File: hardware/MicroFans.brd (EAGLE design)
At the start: 100 x 80 mm, 29 parts, among them IC4 ATMEGA328P, IC7 OPA4251UA, J1 COMPUTER-PERIPHERAL-POWERVERT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, Y1 20Mhz

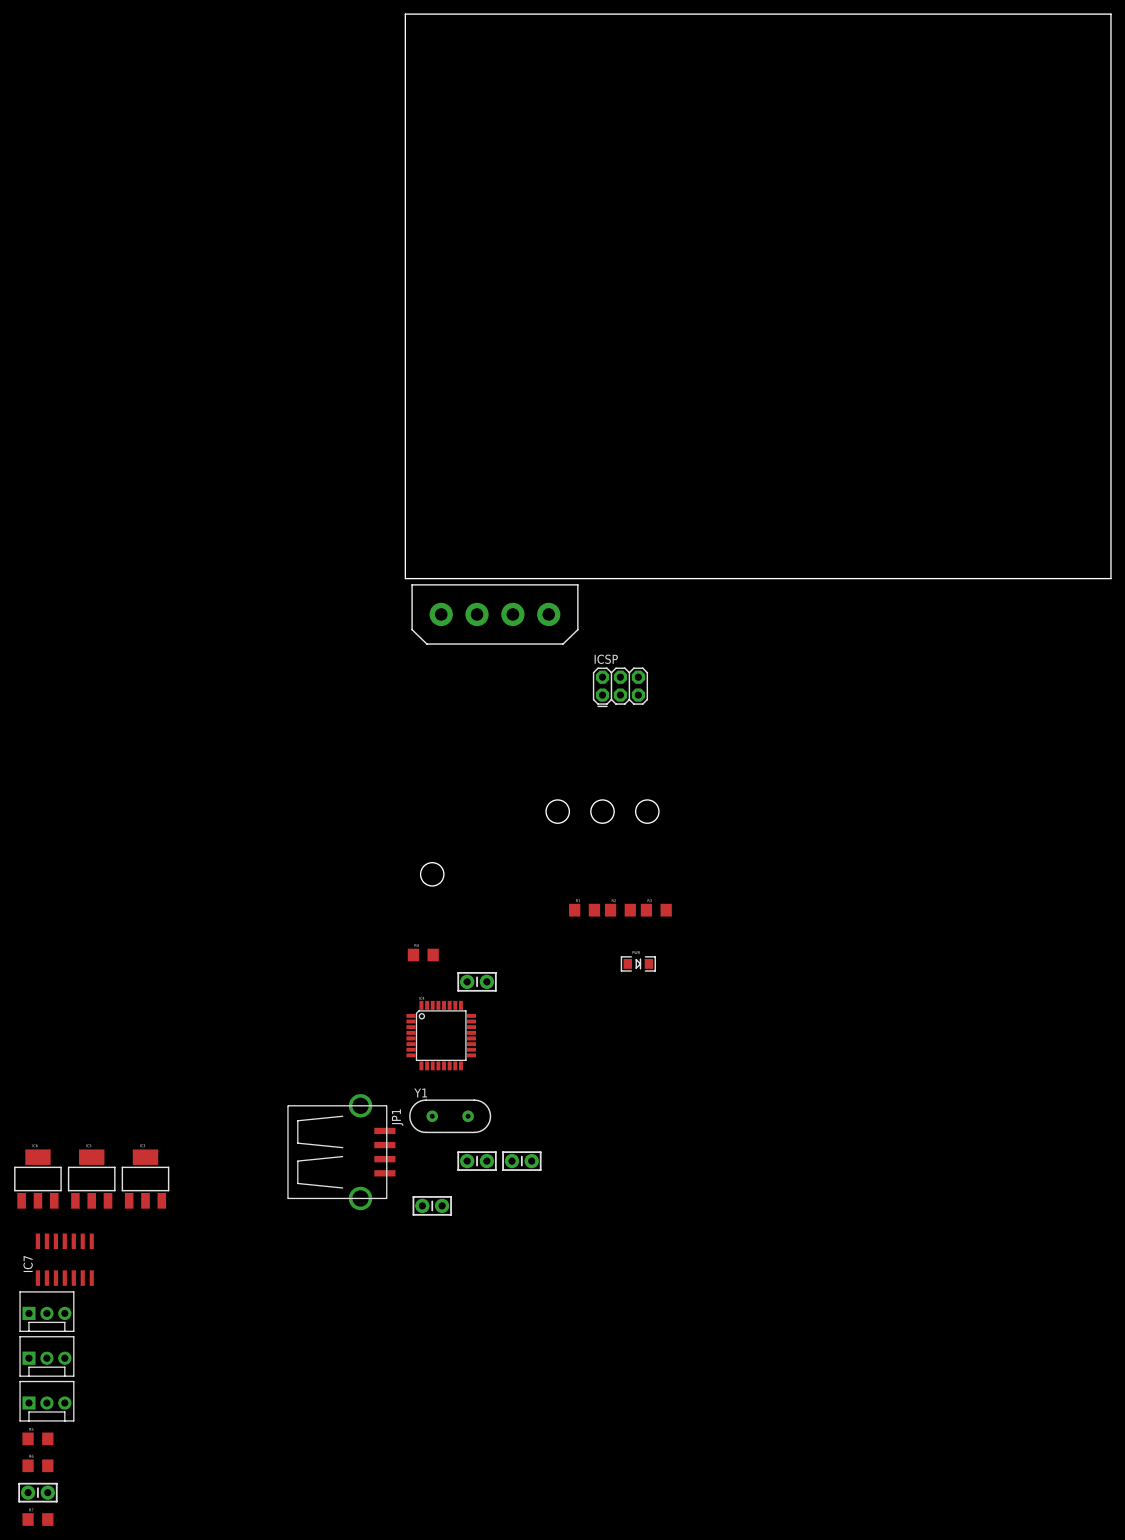
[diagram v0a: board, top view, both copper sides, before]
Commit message: Update board
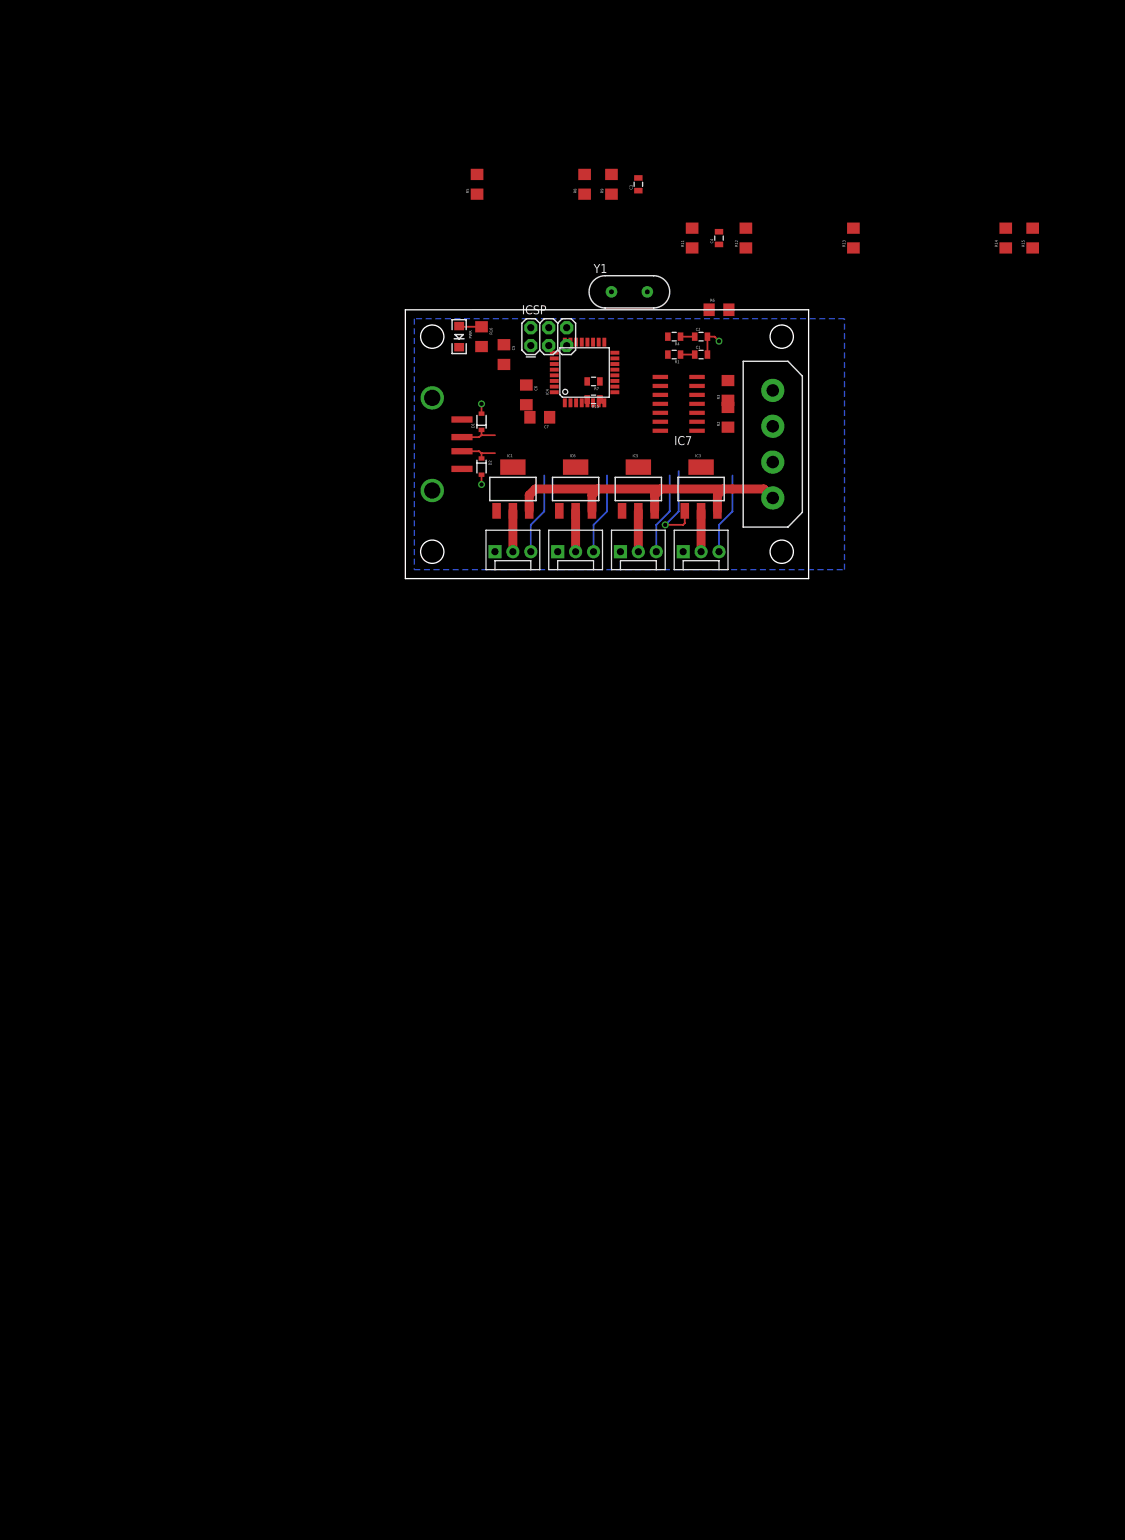
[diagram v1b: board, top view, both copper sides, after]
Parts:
- added C3: 1uF, SparkFun-Capacitors:0805
- added C7: 0.1uF, SparkFun-Passives:1206
- added D1, D2: 3V6, SparkFun-DiscreteSemi:SOD-323
- added IC1: (no value), SparkFun-PowerIC:SOT223
- added JP7: (no value), SparkFun-Connectors:MOLEX-1X3
- added R10: 47K, SparkFun-Passives:0805
- added R11, R8: 8K6, SparkFun-Resistors:1206
- added R12, R9: 2K2, SparkFun-Resistors:1206
- added R13: 1K5, SparkFun-Passives:1206
- added R14, R15: 68, SparkFun-Passives:1206
- added R16: 220, SparkFun-Resistors:1206
- C1, C2: device SparkFun-Capacitors:CAP-PTH-SMALL-KIT -> SparkFun-Capacitors:0805
- C4: value 0.1uF -> 1uF; device SparkFun-Capacitors:CAP-PTH-SMALL-KIT -> SparkFun-Capacitors:0805
- C5, C6: device SparkFun-Capacitors:CAP-PTH-SMALL-KIT -> SparkFun-Passives:1206
- J1: value COMPUTER-PERIPHERAL-POWERVERTICAL -> (none)
- JP1: value USB-A-S -> USB-A-SMD; device SparkFun-Connectors:USB-A-S -> SparkFun-Connectors:USB-A-S-NOSILK-FEMALE
- R1: device SparkFun-Resistors:1206 -> SparkFun-Passives:0805
- R4: value 220 -> 47K; device SparkFun-Resistors:1206 -> SparkFun-Passives:0805
- R6: value 47K -> 2K2
- R7: value 2K2 -> 47K; device SparkFun-Resistors:1206 -> SparkFun-Passives:0805
- Y1: value 20Mhz -> 16MHZ
- moved R6 190.1 mm to (44.5, 38.1)
- moved R5 188.4 mm to (10.2, 55.9), turned to 90 degrees
- moved C1 186.7 mm to (41.9, 31.8)
- moved R7 179.5 mm to (26.7, 27.9), turned to 180 degrees
- moved JP5 152.2 mm to (39.4, 3.81)
- moved IC7 149.3 mm to (38.7, 24.8), turned to 90 degrees
- moved JP4 141.7 mm to (30.5, 3.81)
- moved C4 135.2 mm to (44.5, 48.3), turned to 90 degrees
- moved JP3 131.4 mm to (21.6, 3.81)
- moved IC3 125.6 mm to (41.9, 12.7)
- moved IC5 124.8 mm to (33.0, 12.7)
- moved IC6 124.0 mm to (24.1, 12.7)
- moved Y1 119.6 mm to (31.8, 40.6)
- moved C6 115.7 mm to (17.1, 26.0), turned to 270 degrees
- moved C5 114.3 mm to (14.0, 31.8), turned to 270 degrees
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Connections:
- removed net +25V: IC5.3
- removed net FAN1_TACH: JP5.3
- removed net FAN2_TACH: JP4.3
- removed net FAN3_TACH: JP3.3
- removed net V+: IC7.4
- removed net V-: IC7.11
- new net +12V: IC1.3, IC3.3, IC5.3, IC6.3, IC7.4, J1.12V
- new net N$1: IC1.2, JP7.2
- new net N$19: IC6.1, IC7.14, R8.1
- new net N$20: IC7.13, R8.2, R9.1
- new net N$21: C3.1, IC7.12, R7.1
- new net N$22: IC7.9, R11.2, R12.1
- new net N$23: IC4.25, R7.2
- new net N$24: C4.1, IC7.10, R10.1
- new net N$25: IC1.1, IC7.8, R11.1
- new net N$26: D1.1, JP1.D-, R13.2, R15.1
- new net N$27: JP1.VBUS
- new net N$28: D2.1, JP1.D+, R14.1
- new net N$29: IC4.32, R14.2
- new net N$30: IC4.1, R15.2
- new net N$33: J1.5V, R16.2
- new net N$34: IC4.26, R10.2
- new net SENSE1: IC4.12, JP5.3
- new net SENSE2: IC4.13, JP4.3
- new net SENSE3: IC4.14, JP3.3
- new net SENSE4: IC4.11, JP7.3
- net +5V: now also C7.1, R13.1; no longer C4.1, J1.5V, R4.2
- net GND: now also C1.2, C2.2, C3.2, C7.2, D1.2, D2.2, IC7.11, JP1.GND, JP7.1, R12.2, R6.2, R9.2; no longer R7.2
- net N$12: now also IC4.24, R4.2; no longer R6.2
- net N$13: now also IC6.2, JP3.2; no longer JP4.2
- net N$15: now also C1.1; no longer C2.1
- net N$16: now also R3.1; no longer C2.2, R7.1
- net N$17: now also C2.1, R4.1; no longer C1.1, R6.1
- net N$18: now also R6.1; no longer C1.2, R3.1
- net N$5: now also IC4.23
- net N$7: now also R16.1; no longer R4.1
- net N$8: now also IC5.2, JP4.2; no longer JP3.2
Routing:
- net +12V: track 0.00 -> 48.0 mm
- net N$2: track 0.00 -> 13.0 mm, vias 0 -> 1
- net SENSE2: track 0.00 -> 11.6 mm
- net SENSE4: track 0.00 -> 11.6 mm
- net SENSE3: track 0.00 -> 11.6 mm
- net SENSE1: track 0.00 -> 11.6 mm
- net GND: track 0.00 -> 7.22 mm, vias 0 -> 3
- net N$8: track 0.00 -> 5.79 mm
- net N$31: track 0.00 -> 5.79 mm
- net N$13: track 0.00 -> 5.79 mm
- net N$1: track 0.00 -> 5.79 mm
- net N$28: track 0.00 -> 5.52 mm
- net N$26: track 0.00 -> 5.52 mm
- net N$7: track 0.00 -> 3.22 mm
- net N$17: track 0.00 -> 2.01 mm
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- added copper zone on layer 16, net GND
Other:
- board size 100 x 80 mm -> 57.1 x 38.1 mm
